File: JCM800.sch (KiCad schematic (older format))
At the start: 75 parts, among them U1 ECC83, U2 ECC83, U3 EL84

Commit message: Tweaks
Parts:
- C16: footprint Capacitor_THT:CP_Radial_D8.0mm_P5.00mm -> Capacitor_THT:CP_Radial_D5.0mm_P2.50mm
- R20: footprint Resistor_THT:R_Axial_DIN0411_L9.9mm_D3.6mm_P15.24mm_Horizontal -> Resistor_THT:R_Axial_DIN0414_L11.9mm_D4.5mm_P15.24mm_Horizontal
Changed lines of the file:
@@
 EESchema Schematic File Version 4
-LIBS:JCM800-cache
 EELAYER 30 0
 EELAYER END
@@
 F 0 "C16" H 13818 7246 50  0000 L CNN
 F 1 "22u" H 13818 7155 50  0000 L CNN
-F 2 "Capacitor_THT:CP_Radial_D8.0mm_P5.00mm" H 13738 7050 50  0001 C CNN
+F 2 "Capacitor_THT:CP_Radial_D5.0mm_P2.50mm" H 13738 7050 50  0001 C CNN
 F 3 "~" H 13700 7200 50  0001 C CNN
 	1    13700 7200
@@
 F 0 "R20" H 13080 7154 50  0000 R CNN
 F 1 "220R" H 13080 7245 50  0000 R CNN
-F 2 "Resistor_THT:R_Axial_DIN0411_L9.9mm_D3.6mm_P15.24mm_Horizontal" V 13080 7200 50  0001 C CNN
+F 2 "Resistor_THT:R_Axial_DIN0414_L11.9mm_D4.5mm_P15.24mm_Horizontal" V 13080 7200 50  0001 C CNN
 F 3 "~" H 13150 7200 50  0001 C CNN
 	1    13150 7200

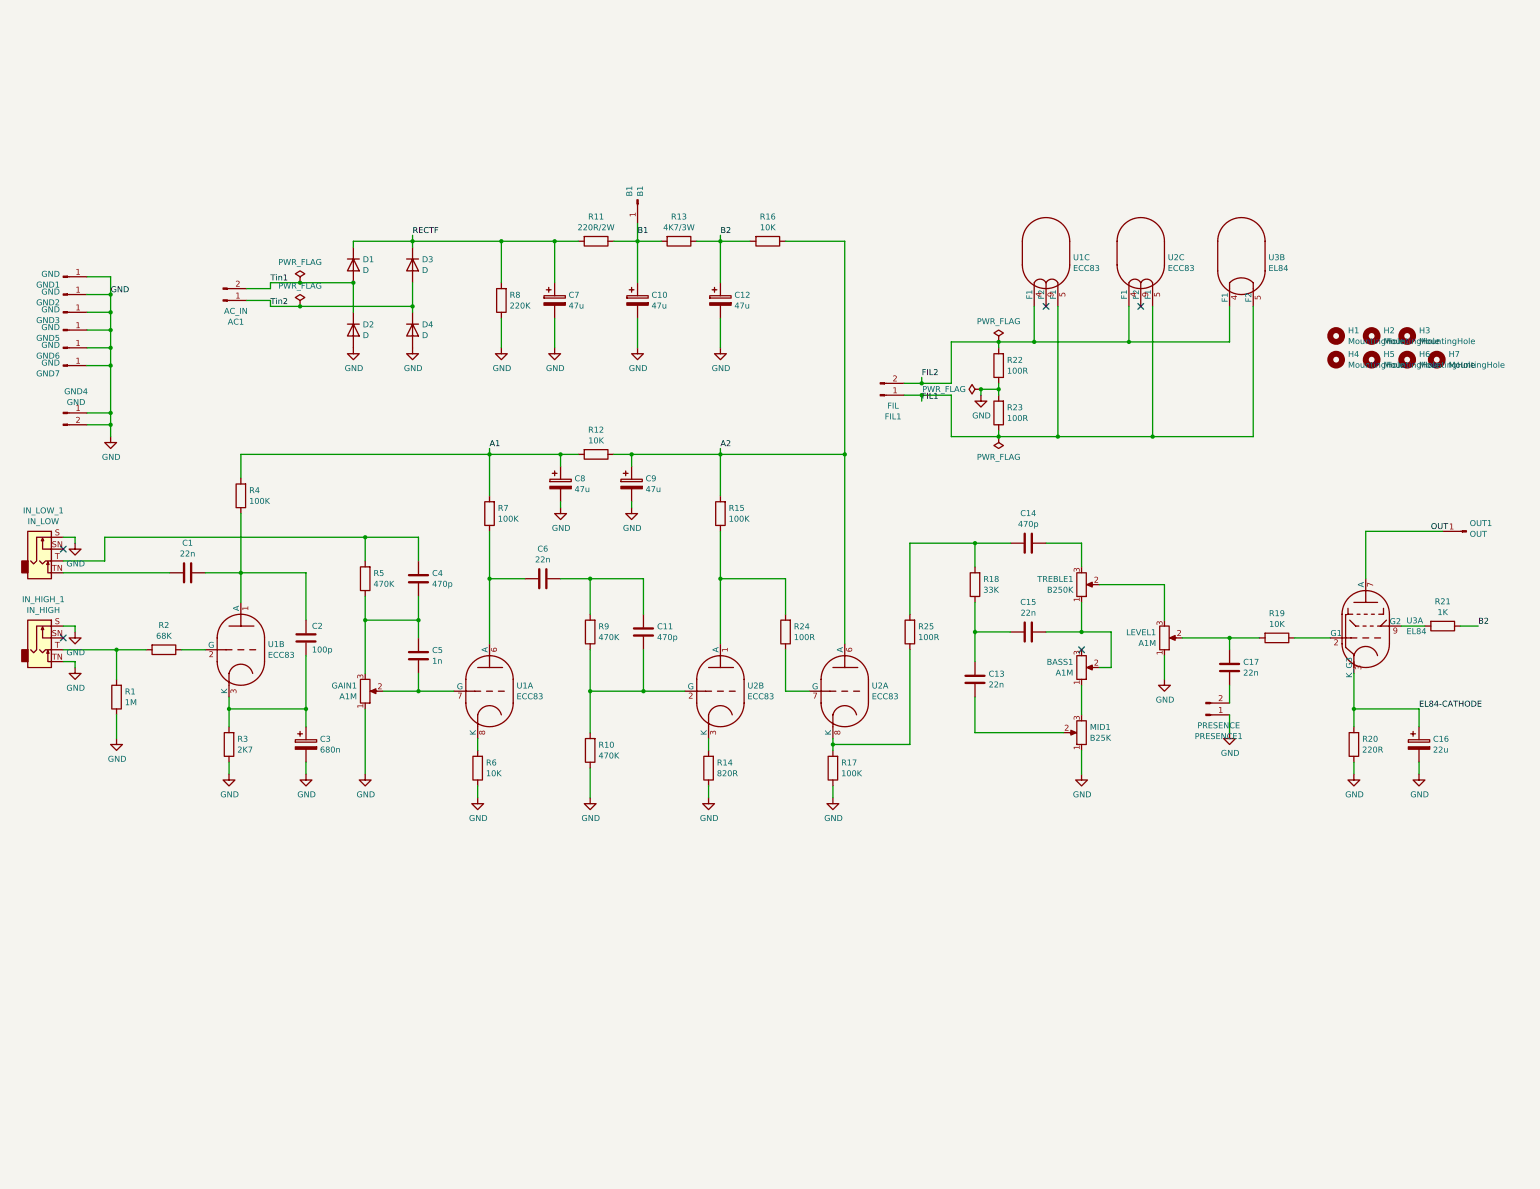
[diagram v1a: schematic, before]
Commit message: Push-Pull branch
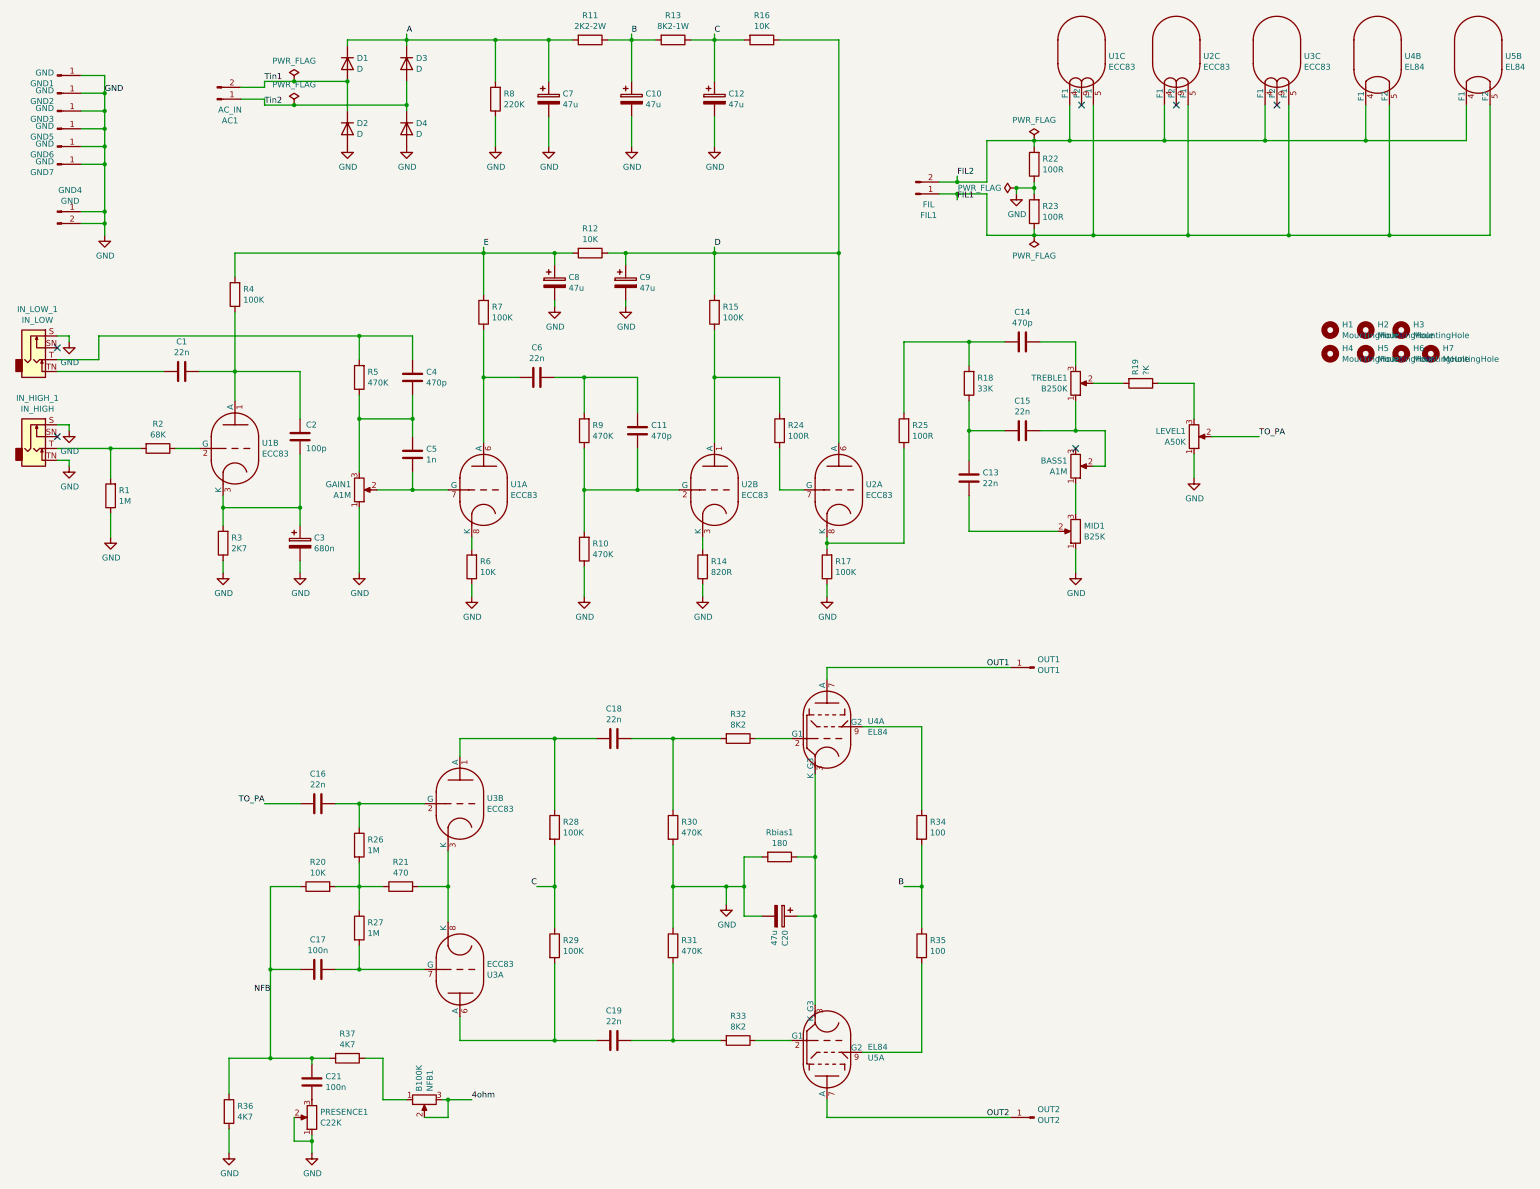
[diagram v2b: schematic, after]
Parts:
- removed B1: B1, Connector_PinHeader_2.54mm:PinHeader_1x01_P2.54mm_Vertical, symbol Connector:Conn_01x01_Male
- removed C16: 22u, Capacitor_THT:CP_Radial_D5.0mm_P2.50mm, symbol Device:CP
- removed PRESENCE1: PRESENCE, TerminalBlock_MetzConnect:TerminalBlock_MetzConnect_Type094_RT03502HBLU_1x02_P5.00mm_Horizontal, symbol Connector:Conn_01x02_Male
- added C16, C18, C19: 22n, Capacitor_THT:C_Rect_L10.3mm_W5.0mm_P7.50mm_MKS4, symbol Device:C
- added C20: 47u, Capacitor_THT:CP_Radial_D7.5mm_P2.50mm, symbol Device:CP
- added C21: 100n, Capacitor_THT:C_Rect_L10.3mm_W5.0mm_P7.50mm_MKS4, symbol Device:C
- added NFB1: B100K, Potentiometer_THT:Potentiometer_Piher_T-16H_Single_Horizontal, symbol Device:R_POT
- added OUT2: OUT2, Connector_PinHeader_2.54mm:PinHeader_1x01_P2.54mm_Vertical, symbol Connector:Conn_01x01_Male
- added PRESENCE1: C22K, Potentiometer_THT:Potentiometer_Piher_T-16H_Single_Horizontal, symbol Device:R_POT
- added R26, R27: 1M, Resistor_THT:R_Axial_DIN0207_L6.3mm_D2.5mm_P10.16mm_Horizontal, symbol Device:R
- added R28, R29: 100K, Resistor_THT:R_Axial_DIN0207_L6.3mm_D2.5mm_P10.16mm_Horizontal, symbol Device:R
- added R30, R31: 470K, Resistor_THT:R_Axial_DIN0207_L6.3mm_D2.5mm_P10.16mm_Horizontal, symbol Device:R
- added R32, R33: 8K2, Resistor_THT:R_Axial_DIN0207_L6.3mm_D2.5mm_P10.16mm_Horizontal, symbol Device:R
- added R34, R35: 100, Resistor_THT:R_Axial_DIN0207_L6.3mm_D2.5mm_P10.16mm_Horizontal, symbol Device:R
- added R36, R37: 4K7, Resistor_THT:R_Axial_DIN0207_L6.3mm_D2.5mm_P10.16mm_Horizontal, symbol Device:R
- added Rbias1: 180, Resistor_THT:R_Axial_DIN0207_L6.3mm_D2.5mm_P10.16mm_Horizontal, symbol Device:R
- added U3: ECC83, tubes:NOVAL, symbol Valve:ECC83
- added U5: EL84, tubes:NOVAL, symbol Valve:EL84
- C17: value 22n -> 100n
- LEVEL1: value A1M -> A50K
- OUT1: value OUT -> OUT1
- R11: value 220R/2W -> 2K2-2W
- R13: value 4K7/3W -> 8K2-1W; footprint Resistor_THT:R_Axial_DIN0617_L17.0mm_D6.0mm_P25.40mm_Horizontal -> Resistor_THT:R_Axial_DIN0414_L11.9mm_D4.5mm_P15.24mm_Horizontal
- R19: value 10K -> ?K
- R20: value 220R -> 10K; footprint Resistor_THT:R_Axial_DIN0414_L11.9mm_D4.5mm_P15.24mm_Horizontal -> Resistor_THT:R_Axial_DIN0207_L6.3mm_D2.5mm_P10.16mm_Horizontal
- R21: value 1K -> 470
- renumbered U3 to U4
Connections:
- net FIL1: now also U3.5 (F1), U5.5 (F2)
- net FIL2: now also U3.4 (F1), U5.4 (F1)
- net GND: now also C20.2, PRESENCE1.1, PRESENCE1.2, R30.2, R31.1, R36.2, Rbias1.2; no longer R20.1
- net NFB: now reaches C17.2
- net NFB: now also R20.1, C21.2, R36.1, R37.2
- net at TREBLE1.2: now also R19.2; no longer LEVEL1.3
- net at R19.1: now also LEVEL1.3; no longer U4.2 (G1)
- net at U4.9 (G2): now also R34.1; no longer R21.2
- net A1 renamed E
- net A2 renamed D
- net B1 renamed B
- net B: now also R34.2, R35.1
- net B2 renamed C
- net C: now also R28.2, R29.1; no longer R21.1
- net EL84-CATHODE: no longer names the net of U4.3 (K_G3)
- net EL84-CATHODE: now also C20.1, Rbias1.1, U5.3 (K_G3); no longer R20.2
- net OUT renamed OUT1
- net RECTF renamed A
- new net: R32.1, U4.2 (G1)
- new net: C18.2, R28.1, U3.1 (A)
- new net: C16.1, R26.1, U3.2 (G)
- new net: R21.2, U3.3 (K), U3.8 (K)
- new net: C19.2, R29.2, U3.6 (A)
- new net: C17.1, R27.2, U3.7 (G)
- new net: R20.2, R21.1, R26.2, R27.1
- new net: C18.1, R30.1, R32.2
- new net: C19.1, R31.2, R33.2
- new net: R33.1, U5.2 (G1)
- new net: R35.2, U5.9 (G2)
- new net: C21.1, PRESENCE1.3
- new net: NFB1.1, R37.1
- new net 4ohm: NFB1.2, NFB1.3
- new net OUT2: OUT2.1 (Pin_1), U5.7 (A)
- new net TO_PA: C16.2, LEVEL1.2
- no-connect marks 5 -> 6
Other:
- moved on the sheet: AC1, BASS1, C1, C10, C11, C12, C13, C14, C15, C2, C3, C4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
